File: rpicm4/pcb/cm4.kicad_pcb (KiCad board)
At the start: 2 copper layers, 85.6 x 55 mm, 3 parts, among them J1 USB_C_Receptacle_USB2.0, J2 USB_C_Receptacle_USB2.0

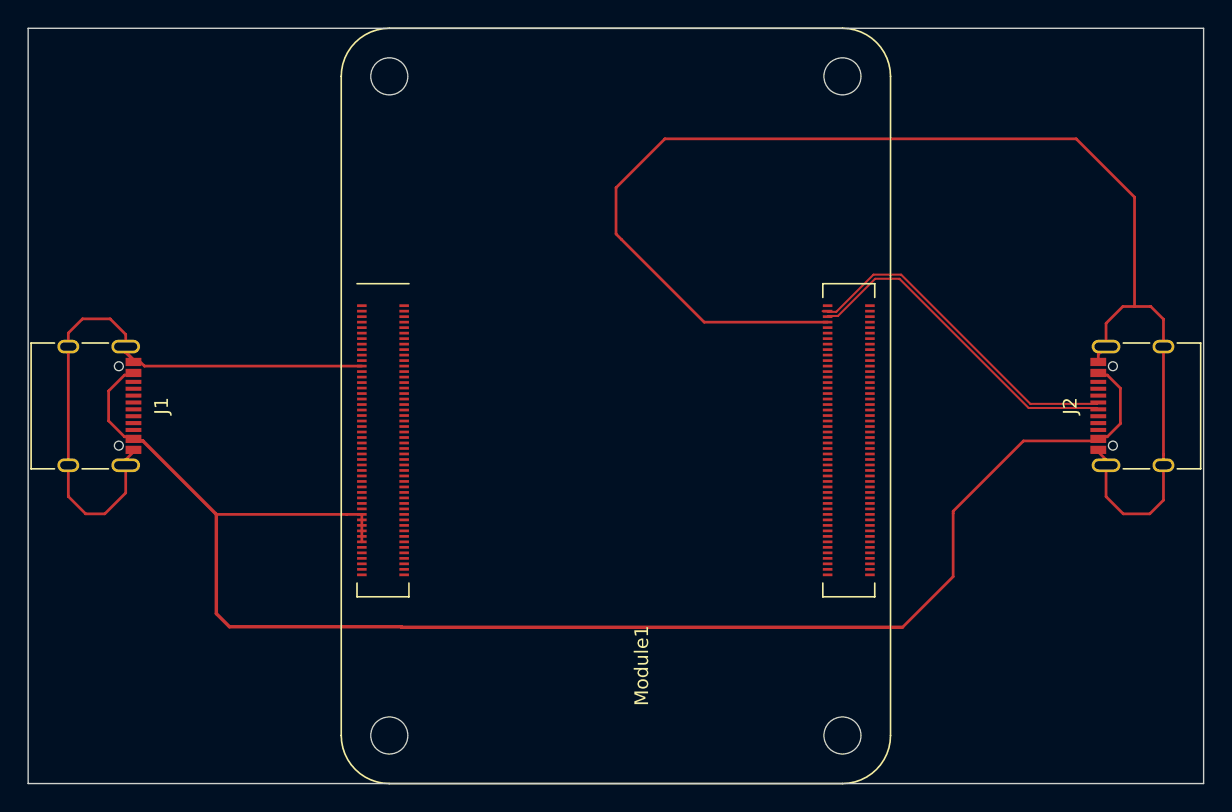
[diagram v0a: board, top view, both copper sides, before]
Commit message: rpicm4 usb
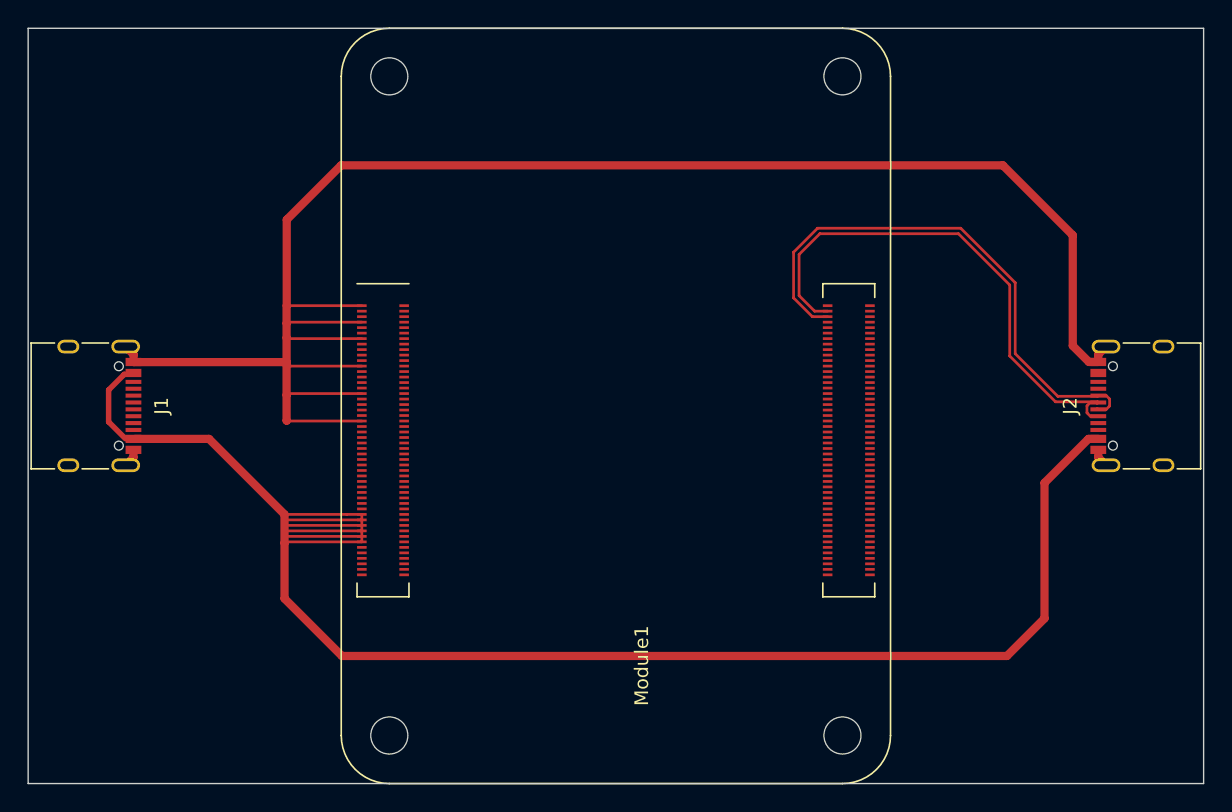
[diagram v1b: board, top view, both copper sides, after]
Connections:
- J2 pad B6: Net-(J2-PadB6) -> /USB_P
- J2 pad B7: Net-(J2-PadB7) -> /USB_N
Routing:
- net +5V: track 114.5 -> 134.3 mm
- net /USB_P: track 24.8 -> 40.0 mm
- net /USB_N: track 25.2 -> 38.7 mm
- net GND: track 144.7 -> 135.4 mm
